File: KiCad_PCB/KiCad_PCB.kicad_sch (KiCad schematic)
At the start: 24 parts, among them J1 530480450, U2 NRF52832-QFAA-R, Y1 ECS-320-8-33B-7KM-TR, Y2 ECS-.327-12.5-12R-TR

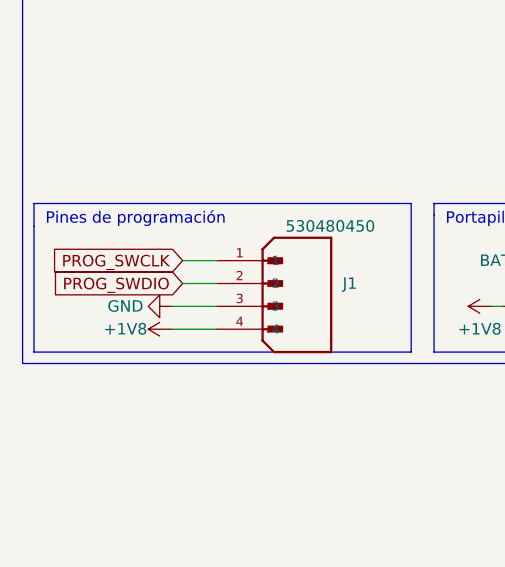
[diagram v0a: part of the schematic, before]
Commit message: Tutorías 10/3
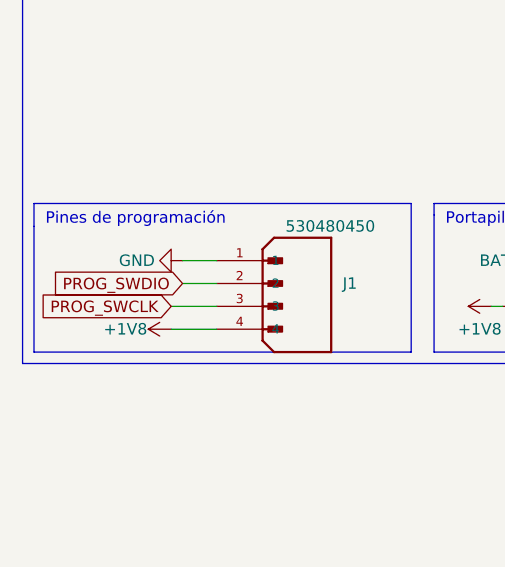
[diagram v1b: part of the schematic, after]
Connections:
- net GND: now also J1.1; no longer J1.3
- net PROG_SWCLK: now also J1.3; no longer J1.1
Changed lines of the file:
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@@
     )
   )
-  (global_label "PROG_SWCLK" (shape input) (at 31.75 130.81 180) (fields_autoplaced)
+  (global_label "PROG_SWCLK" (shape input) (at 30.48 135.89 180) (fields_autoplaced)
     (effects (font (size 1.27 1.27)) (justify right))
-    (property "Intersheet References" "${INTERSHEET_REFS}" (id 0) (at 16.9998 130.7306 0)
+    (property "Intersheet References" "${INTERSHEET_REFS}" (id 0) (at 15.7298 135.8106 0)
       (effects (font (size 1.27 1.27)) (justify right) hide)
     )
@@
     (pin "1")
   )
-  (symbol (lib_id "power:GND") (at 30.48 135.89 270) (unit 1)
-    (in_bom yes) (on_board yes)
-    (property "Reference" "#PWR0126" (id 0) (at 24.13 135.89 0)
-      (effects (font (size 1.27 1.27)) hide)
-    )
-    (property "Value" "GND" (id 1) (at 25.4 135.89 90))
-    (property "Footprint" "" (id 2) (at 30.48 135.89 0)
-      (effects (font (size 1.27 1.27)) hide)
-    )
-    (property "Datasheet" "" (id 3) (at 30.48 135.89 0)
-      (effects (font (size 1.27 1.27)) hide)
-    )
+  (symbol (lib_id "power:GND") (at 31.75 130.81 270) (unit 1)
+    (in_bom yes) (on_board yes)
+    (property "Reference" "#PWR0126" (id 0) (at 25.4 130.81 0)
+      (effects (font (size 1.27 1.27)) hide)
+    )
+    (property "Value" "GND" (id 1) (at 26.67 130.81 90))
+    (property "Footprint" "" (id 2) (at 31.75 130.81 0)
+      (effects (font (size 1.27 1.27)) hide)
+    )
+    (property "Datasheet" "" (id 3) (at 31.75 130.81 0)
+      (effects (font (size 1.27 1.27)) hide)
+    )

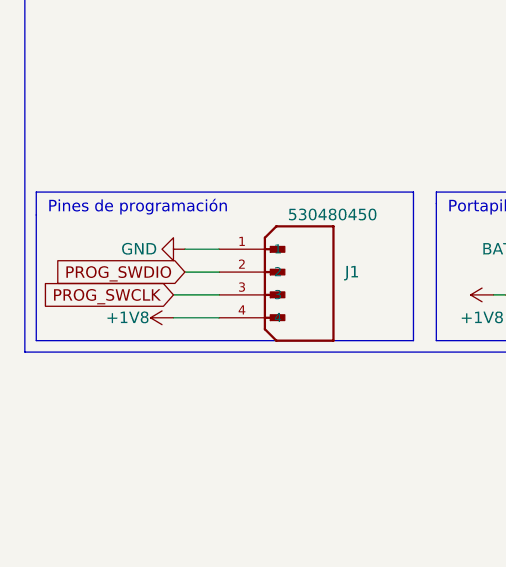
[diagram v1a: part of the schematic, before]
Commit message: Tutoría Modificacion PCB
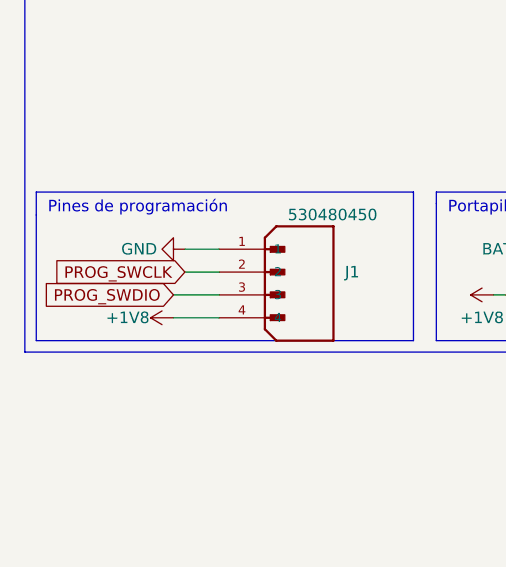
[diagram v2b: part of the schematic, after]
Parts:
- C10, C11, C12, C13, C2, C3, C4, C5, C7, C8, C9: footprint Capacitor_SMD:C_0805_2012Metric -> Capacitor_SMD:C_0603_1608Metric
- R1, R2: footprint Resistor_SMD:R_0805_2012Metric -> Resistor_SMD:R_0603_1608Metric
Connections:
- net PROG_SWCLK: now also J1.2; no longer J1.3
- net PROG_SWDIO: now also J1.3; no longer J1.2
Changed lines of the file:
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@@
     )
   )
-  (global_label "PROG_SWCLK" (shape input) (at 30.48 135.89 180) (fields_autoplaced)
+  (global_label "PROG_SWCLK" (shape input) (at 31.75 133.35 180) (fields_autoplaced)
     (effects (font (size 1.27 1.27)) (justify right))
-    (property "Intersheet References" "${INTERSHEET_REFS}" (id 0) (at 15.7298 135.8106 0)
+    (property "Intersheet References" "${INTERSHEET_REFS}" (id 0) (at 16.9998 133.2706 0)
       (effects (font (size 1.27 1.27)) (justify right) hide)
     )
   )
-  (global_label "PROG_SWDIO" (shape input) (at 31.75 133.35 180) (fields_autoplaced)
+  (global_label "PROG_SWDIO" (shape input) (at 30.48 135.89 180) (fields_autoplaced)
     (effects (font (size 1.27 1.27)) (justify right))
-    (property "Intersheet References" "${INTERSHEET_REFS}" (id 0) (at 17.3626 133.2706 0)
+    (property "Intersheet References" "${INTERSHEET_REFS}" (id 0) (at 16.0926 135.8106 0)
       (effects (font (size 1.27 1.27)) (justify right) hide)
     )
@@
       (effects (font (size 1.27 1.27)) (justify left))
     )
-    (property "Footprint" "Capacitor_SMD:C_0805_2012Metric" (id 2) (at 164.7952 72.39 0)
+    (property "Footprint" "Capacitor_SMD:C_0603_1608Metric" (id 2) (at 164.7952 72.39 0)
       (effects (font (size 1.27 1.27)) hide)
     )
@@
     (property "Reference" "R1" (id 0) (at 154.94 101.6 90))
     (property "Value" "200" (id 1) (at 154.94 106.68 90))
-    (property "Footprint" "Resistor_SMD:R_0805_2012Metric" (id 2) (at 154.94 102.362 90)
+    (property "Footprint" "Resistor_SMD:R_0603_1608Metric" (id 2) (at 154.94 102.362 90)
       (effects (font (size 1.27 1.27)) hide)
     )
@@
       (effects (font (size 1.27 1.27)) (justify left))
     )
-    (property "Footprint" "Capacitor_SMD:C_0805_2012Metric" (id 2) (at 154.6352 45.72 0)
+    (property "Footprint" "Capacitor_SMD:C_0603_1608Metric" (id 2) (at 154.6352 45.72 0)
       (effects (font (size 1.27 1.27)) hide)
     )
@@
       (effects (font (size 1.27 1.27)) (justify left))
     )
-    (property "Footprint" "Capacitor_SMD:C_0805_2012Metric" (id 2) (at 141.9352 45.72 0)
+    (property "Footprint" "Capacitor_SMD:C_0603_1608Metric" (id 2) (at 141.9352 45.72 0)
       (effects (font (size 1.27 1.27)) hide)
     )
@@
     (property "Reference" "C9" (id 0) (at 143.51 62.23 90))
     (property "Value" "100p" (id 1) (at 137.16 62.23 90))
-    (property "Footprint" "Capacitor_SMD:C_0805_2012Metric" (id 2) (at 137.16 61.9252 0)
+    (property "Footprint" "Capacitor_SMD:C_0603_1608Metric" (id 2) (at 137.16 61.9252 0)
       (effects (font (size 1.27 1.27)) hide)
     )
@@
       (effects (font (size 1.27 1.27)) (justify left))
     )
-    (property "Footprint" "Capacitor_SMD:C_0805_2012Metric" (id 2) (at 80.9752 99.06 0)
+    (property "Footprint" "Capacitor_SMD:C_0603_1608Metric" (id 2) (at 80.9752 99.06 0)
       (effects (font (size 1.27 1.27)) hide)
     )
@@
       (effects (font (size 1.27 1.27)) (justify left))
     )
-    (property "Footprint" "Capacitor_SMD:C_0805_2012Metric" (id 2) (at 39.0652 66.04 0)
+    (property "Footprint" "Capacitor_SMD:C_0603_1608Metric" (id 2) (at 39.0652 66.04 0)
       (effects (font (size 1.27 1.27)) hide)
     )
@@
       (effects (font (size 1.27 1.27)) (justify left))
     )
-    (property "Footprint" "Capacitor_SMD:C_0805_2012Metric" (id 2) (at 136.8552 130.81 0)
+    (property "Footprint" "Capacitor_SMD:C_0603_1608Metric" (id 2) (at 136.8552 130.81 0)
       (effects (font (size 1.27 1.27)) hide)
     )
@@
       (effects (font (size 1.27 1.27)) (justify left))
     )
-    (property "Footprint" "Capacitor_SMD:C_0805_2012Metric" (id 2) (at 167.3352 45.72 0)
+    (property "Footprint" "Capacitor_SMD:C_0603_1608Metric" (id 2) (at 167.3352 45.72 0)
       (effects (font (size 1.27 1.27)) hide)
     )
@@
     (property "Reference" "R2" (id 0) (at 133.35 116.84 90))
     (property "Value" "1k" (id 1) (at 133.35 111.76 90))
-    (property "Footprint" "Resistor_SMD:R_0805_2012Metric" (id 2) (at 133.35 112.522 90)
+    (property "Footprint" "Resistor_SMD:R_0603_1608Metric" (id 2) (at 133.35 112.522 90)
       (effects (font (size 1.27 1.27)) hide)
     )
@@
       (effects (font (size 1.27 1.27)) (justify left))
     )
-    (property "Footprint" "Capacitor_SMD:C_0805_2012Metric" (id 2) (at 91.1352 99.06 0)
+    (property "Footprint" "Capacitor_SMD:C_0603_1608Metric" (id 2) (at 91.1352 99.06 0)
       (effects (font (size 1.27 1.27)) hide)
     )
@@
       (effects (font (size 1.27 1.27)) (justify left))
     )
-    (property "Footprint" "Capacitor_SMD:C_0805_2012Metric" (id 2) (at 86.0552 66.04 0)
+    (property "Footprint" "Capacitor_SMD:C_0603_1608Metric" (id 2) (at 86.0552 66.04 0)
       (effects (font (size 1.27 1.27)) hide)
     )
@@
     (property "Reference" "C8" (id 0) (at 143.51 57.15 90))
     (property "Value" "1u" (id 1) (at 138.43 57.15 90))
-    (property "Footprint" "Capacitor_SMD:C_0805_2012Metric" (id 2) (at 137.16 56.8452 0)
+    (property "Footprint" "Capacitor_SMD:C_0603_1608Metric" (id 2) (at 137.16 56.8452 0)
       (effects (font (size 1.27 1.27)) hide)
     )
@@
     )
     (path "/8dc8b5f4-3130-46f4-9c7a-f7056b01dba7"
-      (reference "C2") (unit 1) (value "12p") (footprint "Capacitor_SMD:C_0805_2012Metric")
+      (reference "C2") (unit 1) (value "12p") (footprint "Capacitor_SMD:C_0603_1608Metric")
     )
     (path "/7f1d1afb-649d-4e75-a6b0-5a12cc0a86b8"
-      (reference "C3") (unit 1) (value "12p") (footprint "Capacitor_SMD:C_0805_2012Metric")
+      (reference "C3") (unit 1) (value "12p") (footprint "Capacitor_SMD:C_0603_1608Metric")
     )
     (path "/ba599e5b-50c5-444c-9620-62d56953ce7f"
-      (reference "C4") (unit 1) (value "12p") (footprint "Capacitor_SMD:C_0805_2012Metric")
+      (reference "C4") (unit 1) (value "12p") (footprint "Capacitor_SMD:C_0603_1608Metric")
     )
     (path "/dff3df46-3737-4f7f-a92d-dac2e8871a38"
-      (reference "C5") (unit 1) (value "12p") (footprint "Capacitor_SMD:C_0805_2012Metric")
+      (reference "C5") (unit 1) (value "12p") (footprint "Capacitor_SMD:C_0603_1608Metric")
     )
     (path "/5f4a8894-09c6-4bec-a920-12fe09ca2f55"
-      (reference "C7") (unit 1) (value "100n") (footprint "Capacitor_SMD:C_0805_2012Metric")
+      (reference "C7") (unit 1) (value "100n") (footprint "Capacitor_SMD:C_0603_1608Metric")
     )
     (path "/fca302d0-5c39-47d5-951d-6afa996677a8"
-      (reference "C8") (unit 1) (value "1u") (footprint "Capacitor_SMD:C_0805_2012Metric")
+      (reference "C8") (unit 1) (value "1u") (footprint "Capacitor_SMD:C_0603_1608Metric")
     )
     (path "/608f4001-cff0-46a4-9e8b-63808992aebd"
-      (reference "C9") (unit 1) (value "100p") (footprint "Capacitor_SMD:C_0805_2012Metric")
+      (reference "C9") (unit 1) (value "100p") (footprint "Capacitor_SMD:C_0603_1608Metric")
     )
     (path "/9139e421-b12e-44d5-9237-37af176cd04c"
-      (reference "C10") (unit 1) (value "0.8p") (footprint "Capacitor_SMD:C_0805_2012Metric")
+      (reference "C10") (unit 1) (value "0.8p") (footprint "Capacitor_SMD:C_0603_1608Metric")
     )
     (path "/3c2d2407-2d0c-43bf-9e3d-902b2301426d"
-      (reference "C11") (unit 1) (value "100n") (footprint "Capacitor_SMD:C_0805_2012Metric")
+      (reference "C11") (unit 1) (value "100n") (footprint "Capacitor_SMD:C_0603_1608Metric")
     )
     (path "/0260649a-7e67-4013-a002-9f21265819c7"
-      (reference "C12") (unit 1) (value "100n") (footprint "Capacitor_SMD:C_0805_2012Metric")
+      (reference "C12") (unit 1) (value "100n") (footprint "Capacitor_SMD:C_0603_1608Metric")
     )
     (path "/b41f8a35-424f-4b31-ab71-32800b35b178"
-      (reference "C13") (unit 1) (value "4.7u") (footprint "Capacitor_SMD:C_0805_2012Metric")
+      (reference "C13") (unit 1) (value "4.7u") (footprint "Capacitor_SMD:C_0603_1608Metric")
     )
     (path "/e7837bba-4604-456b-811e-2fbdc4b80544"
@@
     )
     (path "/1d82de6f-ea2b-470a-b75b-09ec0eebcaf1"
-      (reference "R1") (unit 1) (value "200") (footprint "Resistor_SMD:R_0805_2012Metric")
+      (reference "R1") (unit 1) (value "200") (footprint "Resistor_SMD:R_0603_1608Metric")
     )
     (path "/b5190e10-ff79-4359-87b1-0c28e176c29f"
-      (reference "R2") (unit 1) (value "1k") (footprint "Resistor_SMD:R_0805_2012Metric")
+      (reference "R2") (unit 1) (value "1k") (footprint "Resistor_SMD:R_0603_1608Metric")
     )
     (path "/f166b3d3-4633-405d-8711-cb5cdc0e7abc"
